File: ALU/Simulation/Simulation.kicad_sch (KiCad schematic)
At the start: 2 parts

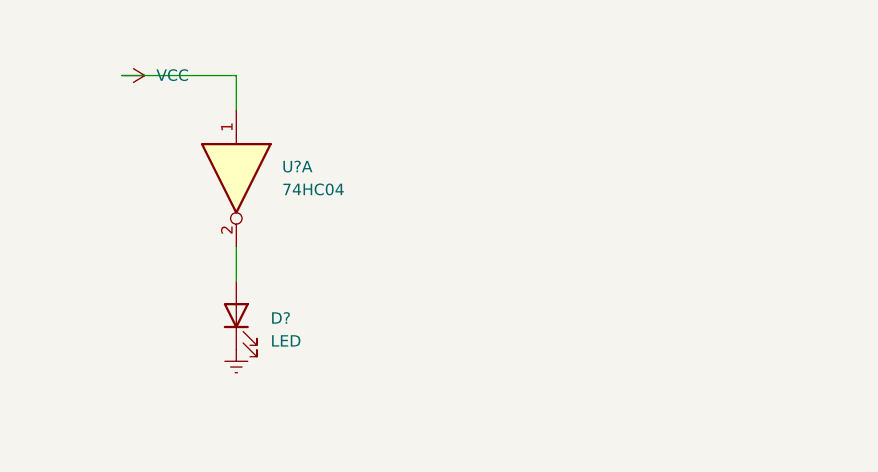
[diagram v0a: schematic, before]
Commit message: Delete files
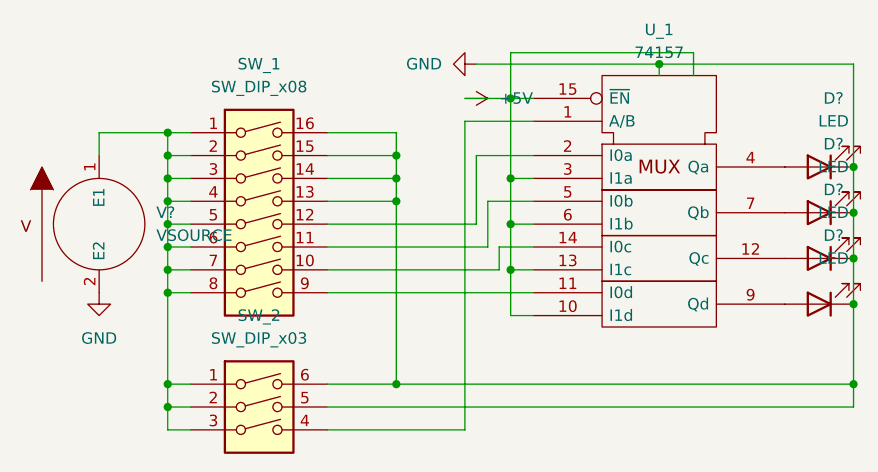
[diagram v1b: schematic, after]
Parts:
- removed D?: LED, symbol Device:LED
- removed U?: 74HC04, symbol 74xx:74HC04
- added D? (x4): LED, symbol Device:LED
- added SW_1: SW_DIP_x08, symbol Switch:SW_DIP_x08
- added SW_2: SW_DIP_x03, symbol Switch:SW_DIP_x03
- added U_1: 74157, symbol 74xx_IEEE:74157
- added V?: VSOURCE, symbol pspice:VSOURCE
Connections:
- new net: SW_1.1, SW_1.2, SW_1.3, SW_1.4, SW_1.5, SW_1.6, SW_1.7, SW_1.8, SW_2.1, SW_2.2, SW_2.3, V?.1 (E1)
- new net: D?.2 (A), U_1.4 (Qa)
- new net: D?.2 (A), U_1.7 (Qb)
- new net: SW_2.4, U_1.1 (A/B)
- new net: D?.2 (A), U_1.9 (Qd)
- new net: D?.2 (A), U_1.12 (Qc)
- new net: SW_1.10, U_1.14 (I0c)
- new net: SW_1.11, U_1.5 (I0b)
- new net: SW_1.12, U_1.2 (I0a)
- new net: SW_1.9, U_1.11 (I0d)
- new net +5V: U_1.10 (I1d), U_1.13 (I1c), U_1.15 (~{EN}), U_1.16 (VCC), U_1.3 (I1a), U_1.6 (I1b)
- new net GND: D?.1 (K), D?.1 (K), D?.1 (K), D?.1 (K), SW_1.13, SW_1.14, SW_1.15, SW_1.16, SW_2.5, SW_2.6, U_1.8 (GND), V?.2 (E2)
